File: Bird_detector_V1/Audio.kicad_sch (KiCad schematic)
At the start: 24 parts, among them U4 TLV320ADC3100, U5 MIC5317, U6 MIC5317

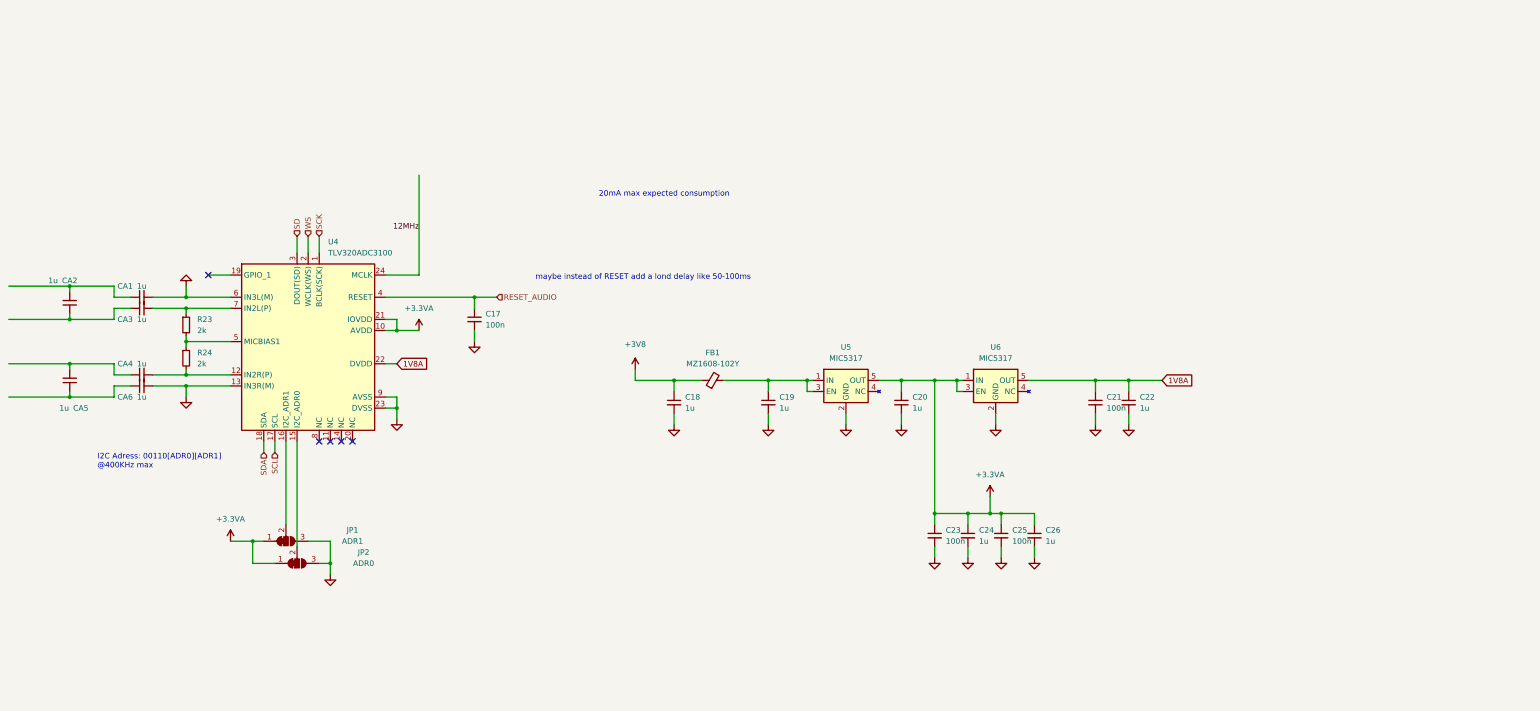
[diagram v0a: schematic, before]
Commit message: j
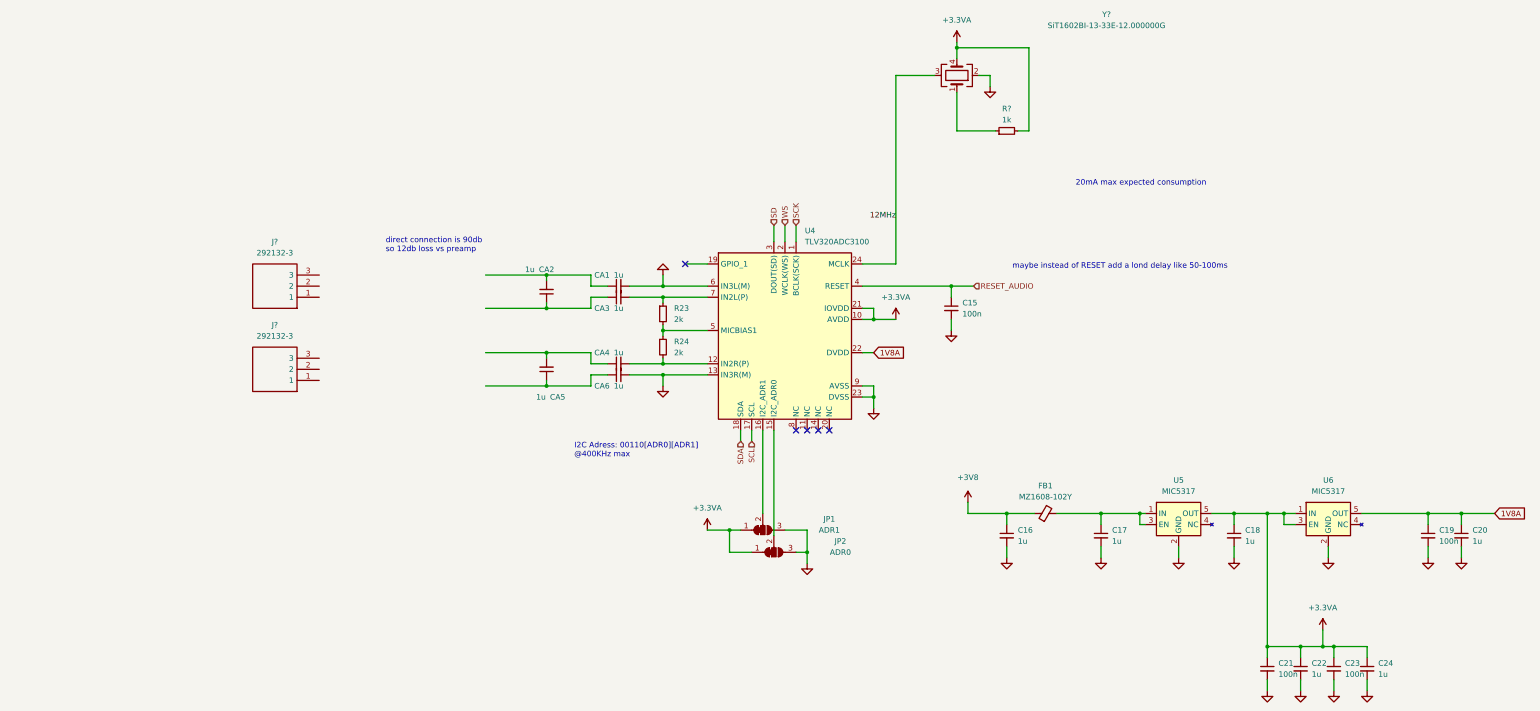
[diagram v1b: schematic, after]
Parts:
- added J? (x2): 292132-3, SHDR3W65P0X200_1X3_780X580X710P, symbol SamacSys_Parts:292132-3
- added R?: 1k, Resistor_SMD:R_0603_1608Metric_Pad0.98x0.95mm_HandSolder, symbol Device:R_Small
- added Y?: SiT1602BI-13-33E-12.000000G, Crystal:Crystal_SMD_2520-4Pin_2.5x2.0mm, symbol Device:Crystal_GND23
- renumbered C17 to C15, C18 to C16, C19 to C17, C20 to C18, C21 to C19, C22 to C20, C23 to C21, C24 to C22, C25 to C23, C26 to C24
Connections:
- net +3.3VA: now also R?.2, Y?.4
- net 12MHz: now also Y?.3
- net GND: now also Y?.2
- new net: R?.1, Y?.1
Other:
- note added: "direct connection is 90db so 12db loss vs preamp"
- moved on the sheet: C15, C16, C17, C18, C19, C20, C21, C22, C23, C24, CA1, CA2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
